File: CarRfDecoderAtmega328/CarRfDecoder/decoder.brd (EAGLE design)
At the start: 98.7 x 80 mm, 52 parts, among them T1 BC847, T2 BC847, T3 IRLML6402, U2 RFM69CW, U3 MCP73831, U4 ATMEGA328P, U6 MIC5219 3.3V, Y1 16MHZ

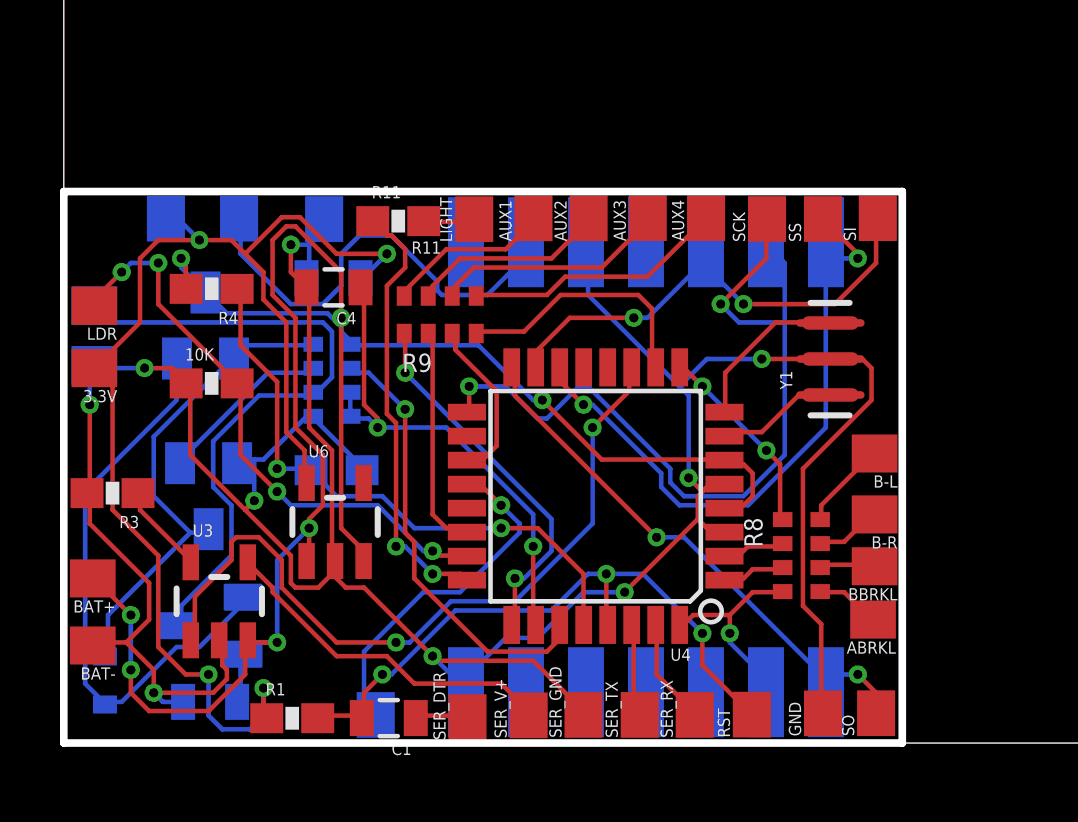
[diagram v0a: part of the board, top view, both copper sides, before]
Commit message: bug fixes and better board routing
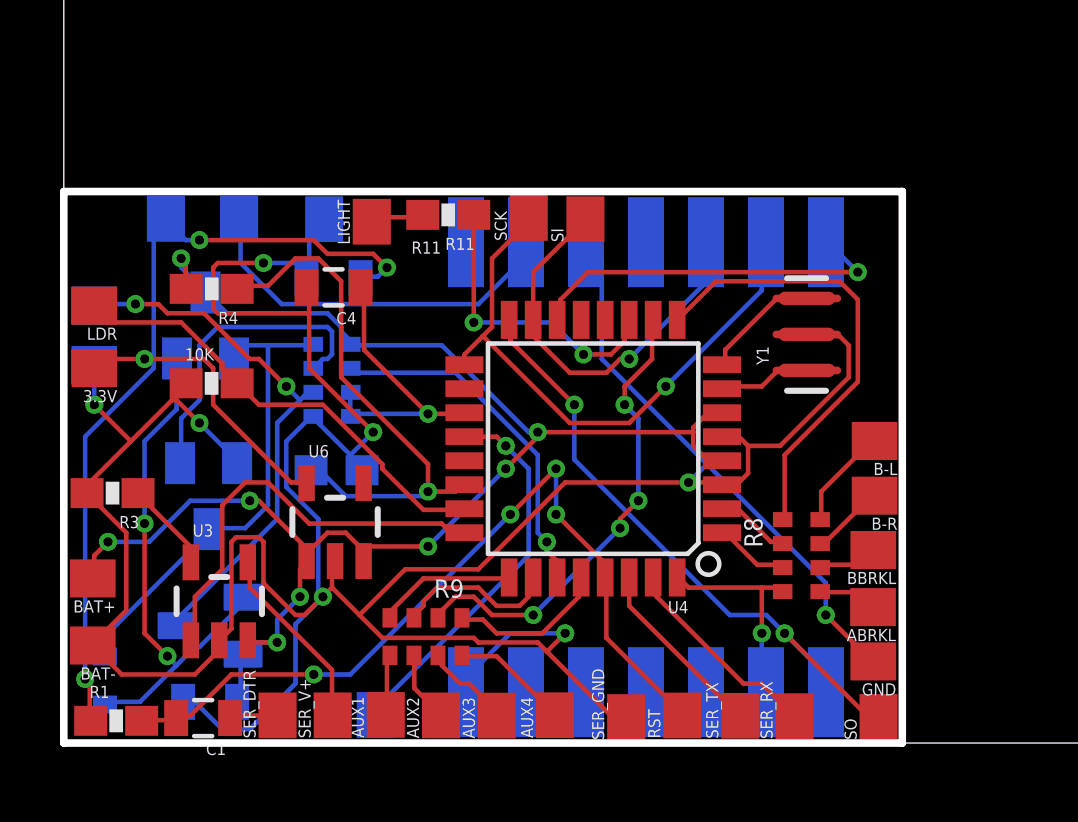
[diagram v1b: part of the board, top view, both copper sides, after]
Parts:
- removed SS: (no value), wirepad:SMD1,27-2,54
- moved AUX3 17.3 mm to (15.7, 0.91)
- moved AUX4 17.3 mm to (17.6, 0.93)
- moved AUX2 17.3 mm to (13.8, 0.92)
- moved AUX1 17.3 mm to (12.0, 0.94)
- moved R9 10.7 mm to (13.3, 3.55), turned to 180 degrees
- moved SI 9.75 mm to (18.7, 17.5)
- moved SCK 7.94 mm to (16.8, 17.5)
- moved SER_V+ 6.53 mm to (10.2, 0.92)
- moved SER_DTR 6.33 mm to (8.40, 0.92)
- moved C1 6.19 mm to (5.92, 0.83)
- moved R1 5.87 mm to (3.02, 0.74)
- moved LIGHT 3.41 mm to (11.5, 17.4)
- moved SER_TX 3.35 mm to (23.8, 0.91)
- moved SER_RX 3.33 mm to (25.6, 0.90)
- moved GND 2.41 mm to (28.3, 2.72), turned to 90 degrees
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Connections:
- removed net AX1: R9.1, U4.25
- removed net AX2: R9.2, U4.22
- removed net AX3: R9.3, U4.19
- removed net AX4: R9.4, U4.10
- removed net N$24: AUX4.1, R9.5
- new net A2: R9.4, U4.25
- new net A6: C4.1, R6.3, R6.4, U4.19
- new net A7: R4.1, R5.2, U4.22
- new net D6: R9.2, U4.10
- new net M: AUX1.1, R9.5
- net A1: now also U3.1; no longer R11.1
- net A3: now also R9.3; no longer C4.1, R6.3, R6.4
- net A5: now also R9.1; no longer R4.1, R5.2
- net D7: now also R11.1; no longer U3.1
- net N$21: now also AUX4.1; no longer AUX1.1
- net N$22: now also AUX3.1; no longer AUX2.1
- net N$23: now also AUX2.1; no longer AUX3.1
- net SS: no longer SS.1
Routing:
- net GND: track 108.4 -> 126.9 mm, vias 9 -> 8
- net A7: track 0.00 -> 18.0 mm, vias 0 -> 1
- net BAT+: track 68.7 -> 52.0 mm, vias 7 -> 8
- net D6: track 0.00 -> 15.7 mm, vias 0 -> 4
- net D7: track 25.4 -> 10.0 mm
- net A5: track 19.9 -> 5.30 mm, vias 2 -> 0
- net AX1: track 12.5 -> 0.00 mm, vias 2 -> 0
- net A3: track 16.9 -> 5.52 mm, vias 2 -> 0
- net A6: track 0.00 -> 9.77 mm, vias 0 -> 1
- net SS: track 22.0 -> 12.5 mm, vias 2 -> 1
- net N$24: track 8.73 -> 0.00 mm
- net BL: track 6.59 -> 15.2 mm, vias 2 -> 0
- net AX4: track 8.59 -> 0.00 mm
- net SCK: track 27.8 -> 19.8 mm, vias 2 -> 1
- net AX2: track 7.52 -> 0.00 mm
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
